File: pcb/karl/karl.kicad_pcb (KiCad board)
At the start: 2 copper layers, 72.4 x 57.1 mm, 30 parts, among them J1 Raspberry_Pi, J2 Power, J3 Battery, J4 LIDAR_Power, J5 Motor_Power, Q1 MMBT3904, Q2 MMBT3904, U1 MCP3421A0T-ECH

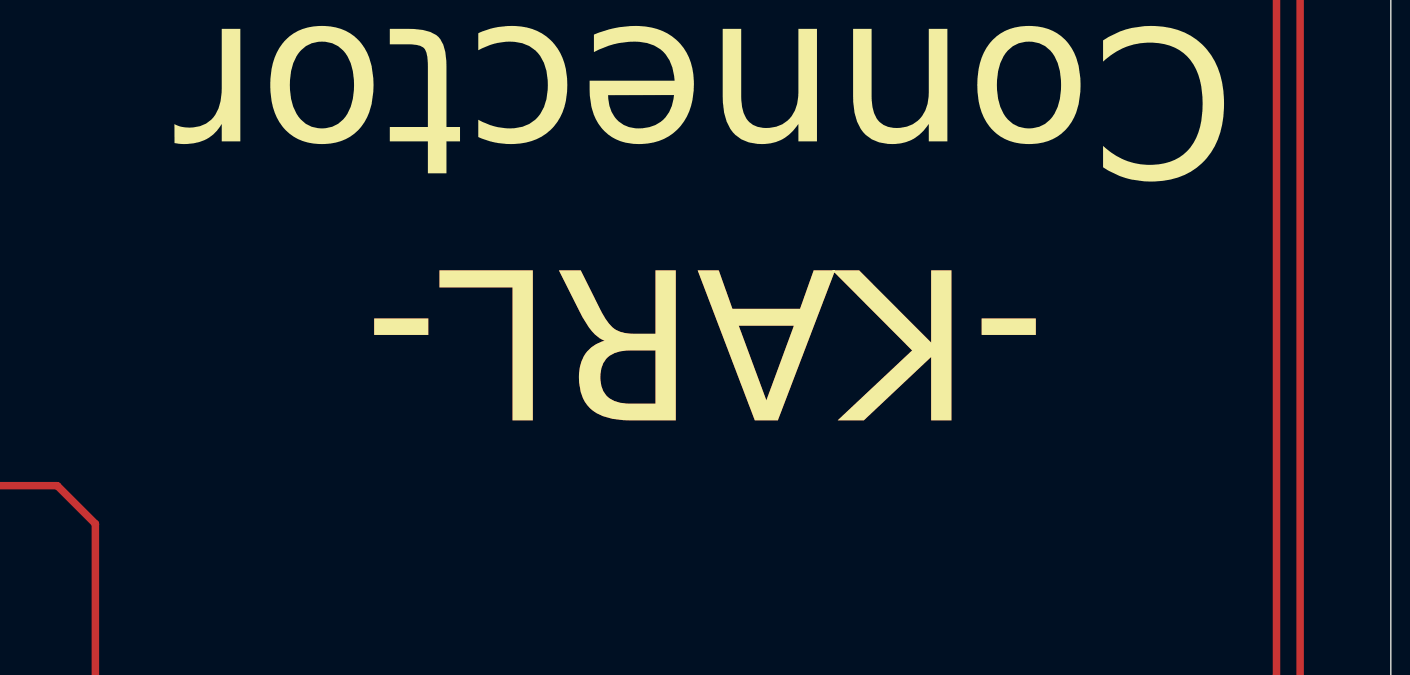
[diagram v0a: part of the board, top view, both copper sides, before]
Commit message: saved
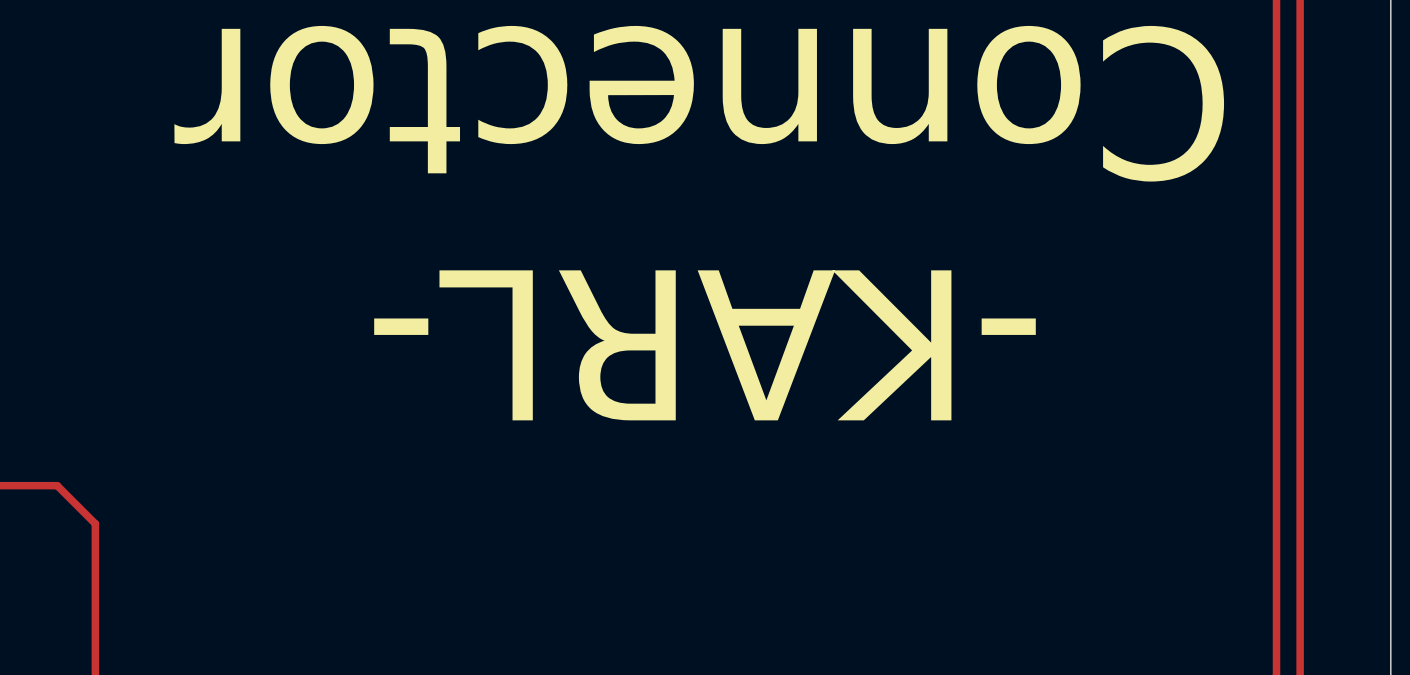
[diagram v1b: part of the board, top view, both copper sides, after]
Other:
- board text removed: "-KARL-"
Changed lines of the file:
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@@
   (general
     (thickness 1.6)
-    (drawings 18)
+    (drawings 17)
     (tracks 197)
     (zones 0)
@@
     (effects (font (size 1.5 1.5) (thickness 0.3)) (justify left))
   )
-  (gr_text "-KARL-\n " (at 76.2 44.45 180) (layer F.Cu)
-    (effects (font (size 5 5) (thickness 0.6)))
-  )
   (gr_text "c Manuel Fehren" (at 73.66 21.59 180) (layer F.SilkS)
